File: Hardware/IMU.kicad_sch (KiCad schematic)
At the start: 1 part, among them U4 ICM-20948

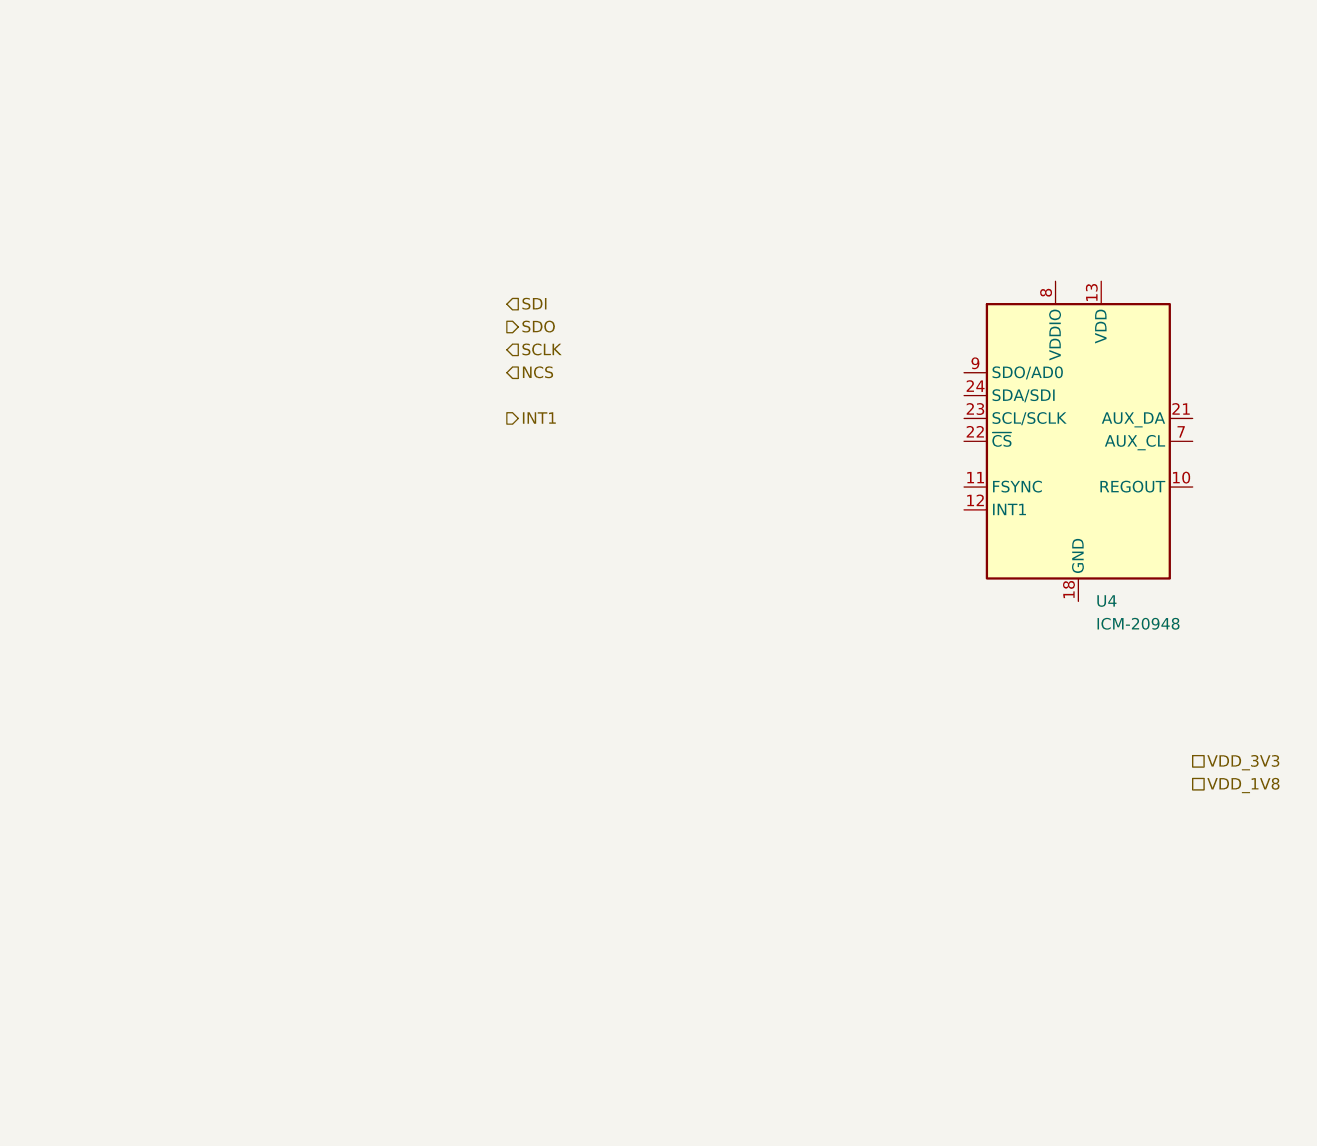
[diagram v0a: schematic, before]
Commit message: Checkpoint
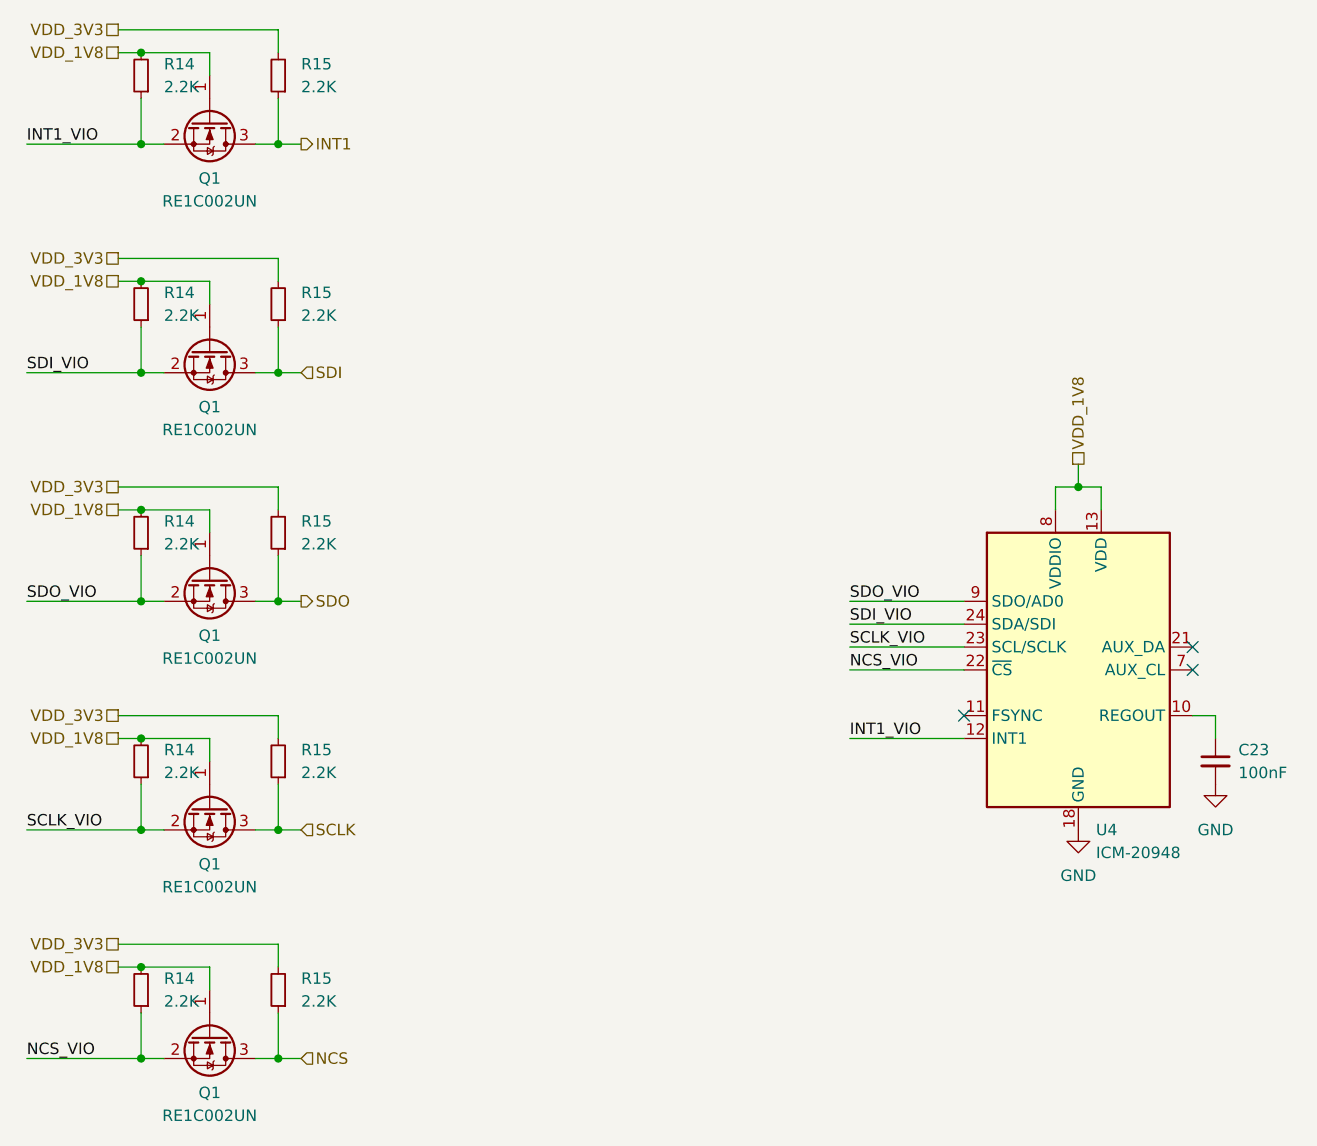
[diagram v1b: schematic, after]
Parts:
- added C23: 100nF, symbol Device:C_Small
- added Q1 (x5): RE1C002UN, Package_TO_SOT_SMD:SOT-416, symbol Device:Q_NMOS_GSD
- added R14 (x5), R15 (x5): 2.2K, symbol Device:R_Small
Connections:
- net INT1: now also Q1.3 (D), R15.1
- net NCS: now also Q1.3 (D), R15.1
- net SCLK: now also Q1.3 (D), R15.1
- net SDI: now also Q1.3 (D), R15.1
- net SDO: now also Q1.3 (D), R15.1
- net VDD_1V8: now also U4.13 (VDD), U4.8 (VDDIO), Q1.1 (G), Q1.1 (G), Q1.1 (G), Q1.1 (G), Q1.1 (G), R14.2, R14.2, R14.2, R14.2, R14.2
- net VDD_3V3: now also R15.2, R15.2, R15.2, R15.2, R15.2
- net at U4.10 (REGOUT): now also C23.1
- net INT1_VIO: now reaches U4.12 (INT1)
- net INT1_VIO: now also Q1.2 (S), R14.1
- net GND: now reaches U4.18 (GND), U4.20 (GND)
- net GND: now also C23.2
- net NCS_VIO: now reaches U4.22 (~{CS})
- net NCS_VIO: now also Q1.2 (S), R14.1
- net SCLK_VIO: now reaches U4.23 (SCL/SCLK)
- net SCLK_VIO: now also Q1.2 (S), R14.1
- net SDI_VIO: now reaches U4.24 (SDA/SDI)
- net SDI_VIO: now also Q1.2 (S), R14.1
- net SDO_VIO: now reaches U4.9 (SDO/AD0)
- net SDO_VIO: now also Q1.2 (S), R14.1
- no-connect marks 0 -> 3
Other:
- moved on the sheet: U4
